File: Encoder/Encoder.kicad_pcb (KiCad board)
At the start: 2 copper layers, 158.6 x 85.2 mm, 52 parts, among them J1 Conn_01x02_Socket, J2 Conn_01x02_Socket, J3 Conn_01x04_Socket, U1 TL072, U2 TL072, U3 TL072

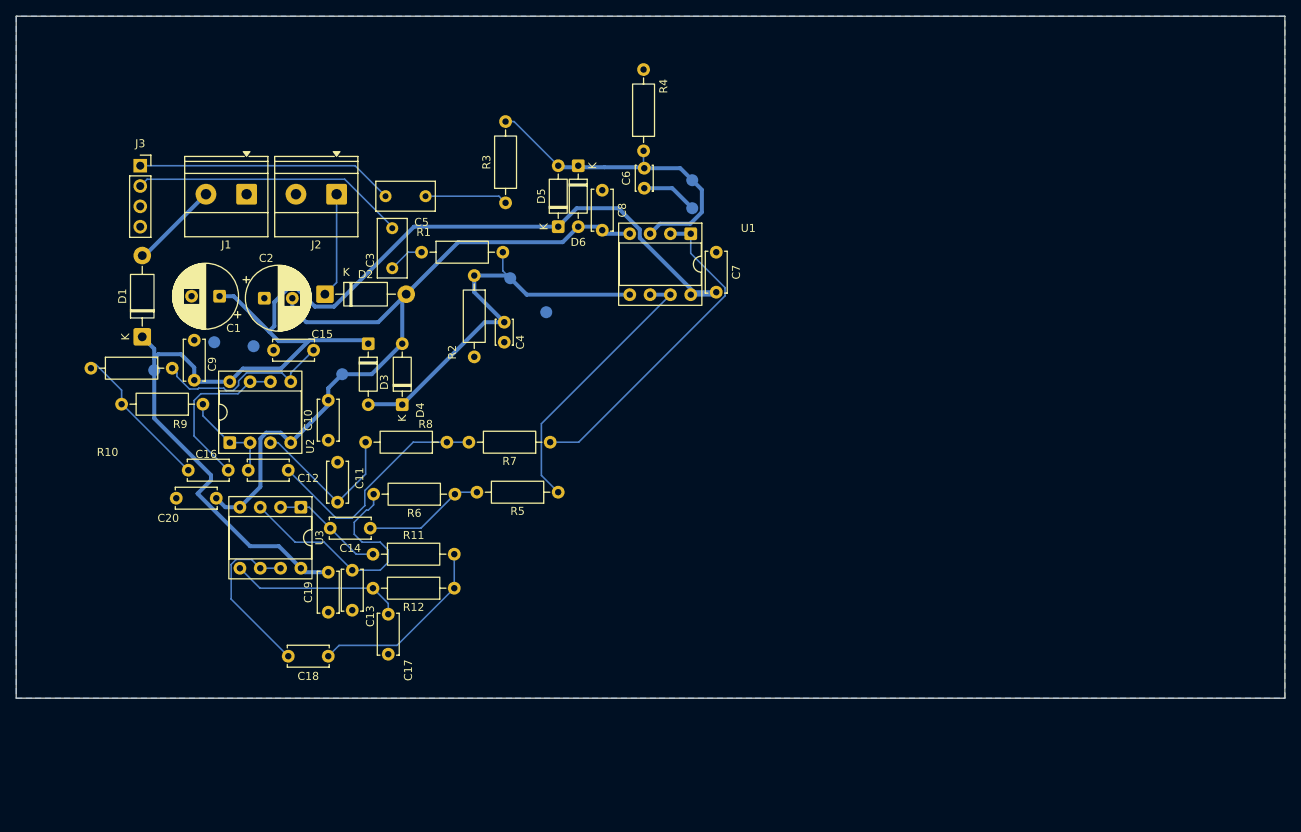
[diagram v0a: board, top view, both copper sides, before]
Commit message: new board layout
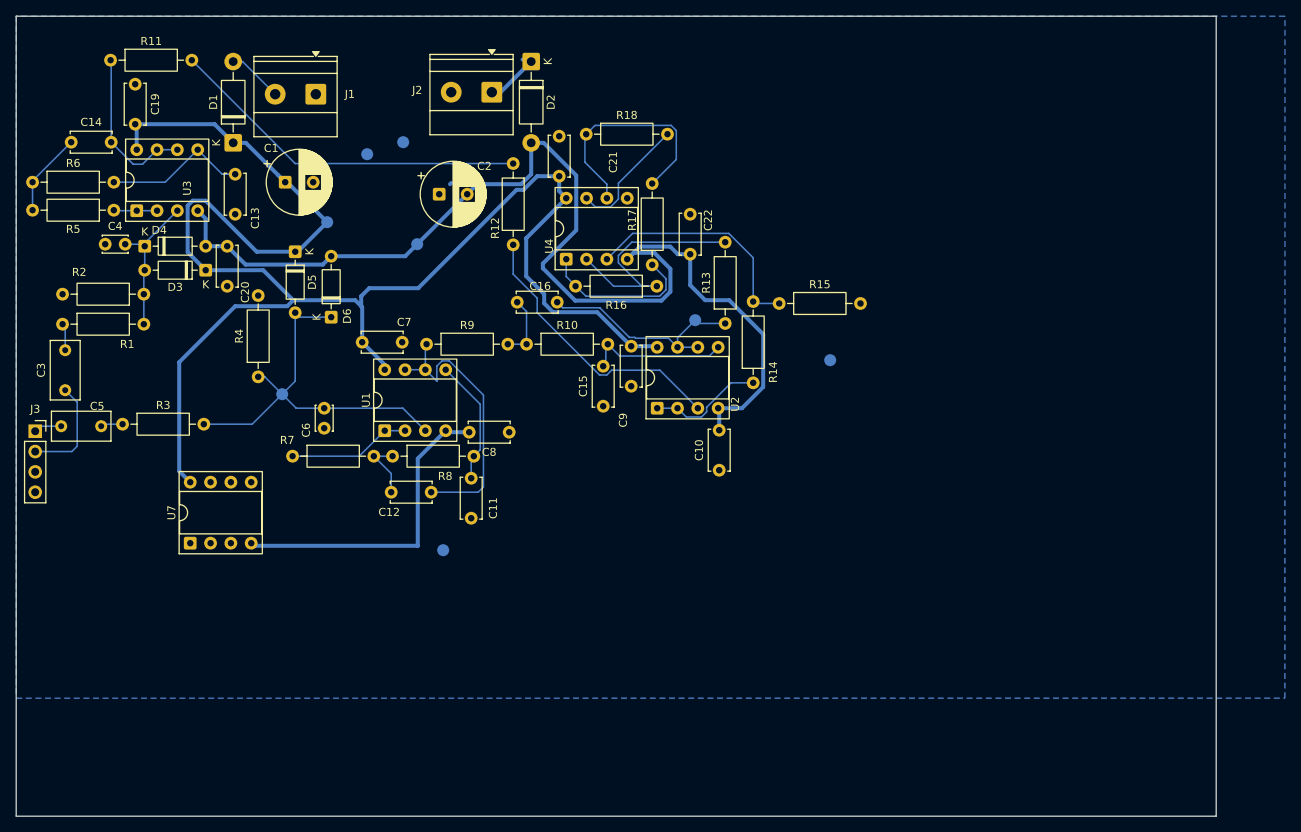
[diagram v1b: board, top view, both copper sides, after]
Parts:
- removed C17: 330 p, Capacitor_THT:C_Disc_D5.0mm_W2.5mm_P5.00mm
- removed C18: 2.2 n, Capacitor_THT:C_Disc_D5.0mm_W2.5mm_P5.00mm
- removed TP_GND2, TP_R1: TestPoint, TestPoint:TestPoint_Pad_D1.5mm
- added C21: 100n, Capacitor_THT:C_Disc_D5.0mm_W2.5mm_P5.00mm, F.Cu at (79.9, 27.0)
- added C22: 100n, Capacitor_THT:C_Disc_D5.0mm_W2.5mm_P5.00mm, F.Cu at (96.2, 36.8)
- added R13: 100k, Resistor_THT:R_Axial_DIN0207_L6.3mm_D2.5mm_P10.16mm_Horizontal, F.Cu at (100.6, 50.4)
- added R14: 100k, Resistor_THT:R_Axial_DIN0207_L6.3mm_D2.5mm_P10.16mm_Horizontal, F.Cu at (104.1, 57.8)
- added R15: 100k, Resistor_THT:R_Axial_DIN0207_L6.3mm_D2.5mm_P10.16mm_Horizontal, F.Cu at (107.4, 47.9)
- added R16: 100k, Resistor_THT:R_Axial_DIN0207_L6.3mm_D2.5mm_P10.16mm_Horizontal, F.Cu at (92.1, 45.8)
- added R17: 100k, Resistor_THT:R_Axial_DIN0207_L6.3mm_D2.5mm_P10.16mm_Horizontal, F.Cu at (91.5, 43.1)
- added R18: 100k, Resistor_THT:R_Axial_DIN0207_L6.3mm_D2.5mm_P10.16mm_Horizontal, F.Cu at (83.2, 26.8)
- added TP_GND5: TestPoint, TestPoint:TestPoint_Pad_D1.5mm, B.Cu at (113.8, 55.0)
- added TP_L2: TestPoint, TestPoint:TestPoint_Pad_D1.5mm, B.Cu at (96.9, 50.0)
- added U4: TL072, Package_DIP:DIP-8_W7.62mm_Socket, F.Cu at (80.8, 42.4)
- added U7: TL072, Package_DIP:DIP-8_W7.62mm_Socket, F.Cu at (33.8, 77.9)
- moved C19 70.3 mm to (26.9, 20.5), turned to -90 degrees
- moved R11 69.9 mm to (23.8, 17.5)
- moved R5 65.8 mm to (24.2, 36.2)
- moved R6 65.6 mm to (14.0, 32.8), turned to 0 degrees
- moved C14 61.0 mm to (18.9, 27.8), turned to 0 degrees
- moved TP_L1 57.8 mm to (45.2, 59.2), turned to 180 degrees
- moved R4 55.8 mm to (42.2, 57.1)
- moved R3 55.3 mm to (25.3, 63.0), turned to 0 degrees
- moved C9 54.9 mm to (88.9, 58.2), turned to 90 degrees
- moved R10 54.5 mm to (75.8, 53.0)
- moved U2 53.6 mm to (92.1, 61.0)
- moved R12 53.6 mm to (74.1, 30.4), turned to -90 degrees
- moved TP_GND4 52.9 mm to (65.4, 78.8), turned to 180 degrees
- moved C13 51.6 mm to (39.4, 36.8)
- moved C4 51.4 mm to (23.1, 40.5), turned to 0 degrees
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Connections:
- C11 pad 2: Net-(U2A-+) -> Net-(U1B-+)
- C12 pad 2: Net-(U2A--) -> Net-(U1B--)
- C13 pad 2: Net-(U3A-+) -> Net-(U3B-+)
- C14 pad 2: Net-(U3A--) -> Net-(U3B--)
- R11 pad 1: Net-(U3A--) -> Net-(U3B--)
- R12 pad 2: Net-(U3B-+) -> Net-(U2A-+)
- R5 pad 1: Net-(U1B--) -> Net-(U3A--)
- R6 pad 2: Net-(U3A-+) -> Net-(U3B-+)
- R8 pad 2: Net-(U2A-+) -> Net-(U1B-+)
- R9 pad 1: Net-(U2A--) -> Net-(U1B--)
- U1 pad 5: /right -> Net-(U1B-+)
- U3 pad 3: Net-(U3A-+) -> /right
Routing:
- net -9V: track 94.5 -> 183.9 mm
- net /right: track 52.8 -> 18.5 mm
- net Net-(U3A-+): track 32.4 -> 0.00 mm
- net Net-(U4A--): track 0.00 -> 31.2 mm
- net +9V: track 163.6 -> 194.7 mm
- net Net-(U4A-+): track 0.00 -> 29.7 mm
- net Net-(U4B--): track 0.00 -> 29.1 mm
- net Net-(J3-Pin_1): track 32.2 -> 3.51 mm
- net Net-(U1A--): track 41.5 -> 15.4 mm
- net Net-(C12-Pad1): track 30.1 -> 7.74 mm
- net Net-(C18-Pad1): track 23.5 -> 45.5 mm
- net Net-(J3-Pin_2): track 34.5 -> 13.1 mm
- net Net-(R16-Pad2): track 0.00 -> 19.8 mm
- net Net-(U1B-+): track 0.00 -> 15.8 mm
- net Net-(R18-Pad2): track 0.00 -> 15.5 mm
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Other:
- board size 158.6 x 85.2 mm -> 150 x 100 mm

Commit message: encoder pcb test 1 is almost done
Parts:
- removed the U2 at (92.1, 61.0)
- removed U7: TL072, Package_DIP:DIP-8_W7.62mm_Socket
- added C17: 2.2n, Capacitor_THT:C_Disc_D5.0mm_W2.5mm_P5.00mm, F.Cu at (142.2, 113.8)
- added C18: 100n, Capacitor_THT:C_Disc_D5.0mm_W2.5mm_P5.00mm, F.Cu at (134.9, 113.8)
- added C23: 1 n, Capacitor_THT:C_Disc_D5.0mm_W2.5mm_P5.00mm, F.Cu at (58.0, 57.2)
- added C24: 1 n, Capacitor_THT:C_Disc_D5.0mm_W2.5mm_P5.00mm, F.Cu at (65.8, 64.2)
- added C25: 1 n, Capacitor_THT:C_Disc_D5.0mm_W2.5mm_P5.00mm, F.Cu at (77.4, 94.7)
- added C26: 1 n, Capacitor_THT:C_Disc_D5.0mm_W2.5mm_P5.00mm, F.Cu at (67.5, 94.5)
- added C27: 100n, Capacitor_THT:C_Disc_D5.0mm_W2.5mm_P5.00mm, F.Cu at (128.0, 132.2)
- added C28: 100n, Capacitor_THT:C_Disc_D5.0mm_W2.5mm_P5.00mm, F.Cu at (112.2, 120.1)
- added C29: 100n, Capacitor_THT:C_Disc_D5.0mm_W2.5mm_P5.00mm, F.Cu at (101.6, 94.1)
- added C30: 100n, Capacitor_THT:C_Disc_D5.0mm_W2.5mm_P5.00mm, F.Cu at (116.0, 97.4)
- added C31: 330 p, Capacitor_THT:C_Disc_D5.0mm_W2.5mm_P5.00mm, F.Cu at (99.1, 53.2)
- added C32: 2.2 n, Capacitor_THT:C_Disc_D5.0mm_W2.5mm_P5.00mm, F.Cu at (74.2, 68.0)
- added C33: 330 p, Capacitor_THT:C_Disc_D5.0mm_W2.5mm_P5.00mm, F.Cu at (90.5, 80.8)
- added C34: 2.2 n, Capacitor_THT:C_Disc_D5.0mm_W2.5mm_P5.00mm, F.Cu at (78.2, 91.5)
- added C35: 3.3n, Capacitor_THT:C_Disc_D5.0mm_W2.5mm_P5.00mm, F.Cu at (146.1, 86.6)
- added C36: 220P, Capacitor_THT:C_Disc_D5.0mm_W2.5mm_P5.00mm, F.Cu at (146.2, 110.7)
- added C37: 100n, Capacitor_THT:C_Disc_D5.0mm_W2.5mm_P5.00mm, F.Cu at (128.5, 70.1)
- added C38: 100n, Capacitor_THT:C_Disc_D5.0mm_W2.5mm_P5.00mm, F.Cu at (125.8, 82.4)
- added C39: 100n, Capacitor_THT:C_Disc_D5.0mm_W2.5mm_P5.00mm, F.Cu at (129.0, 62.5)
- added C40: 100n, Capacitor_THT:C_Disc_D5.0mm_W2.5mm_P5.00mm, F.Cu at (126.3, 102.8)
- added C41: 100n, Capacitor_THT:C_Disc_D5.0mm_W2.5mm_P5.00mm, F.Cu at (132.6, 67.4)
- added R19: 100k, Resistor_THT:R_Axial_DIN0207_L6.3mm_D2.5mm_P10.16mm_Horizontal, F.Cu at (76.9, 72.8)
- added R20: 100k, Resistor_THT:R_Axial_DIN0207_L6.3mm_D2.5mm_P10.16mm_Horizontal, F.Cu at (82.9, 78.0)
- added R21: 100k, Resistor_THT:R_Axial_DIN0207_L6.3mm_D2.5mm_P10.16mm_Horizontal, F.Cu at (106.8, 78.3)
- added R22: 100k, Resistor_THT:R_Axial_DIN0207_L6.3mm_D2.5mm_P10.16mm_Horizontal, F.Cu at (94.8, 107.8)
- added R23: 100k, Resistor_THT:R_Axial_DIN0207_L6.3mm_D2.5mm_P10.16mm_Horizontal, F.Cu at (90.2, 107.7)
- added R24: 100k, Resistor_THT:R_Axial_DIN0207_L6.3mm_D2.5mm_P10.16mm_Horizontal, F.Cu at (109.4, 81.0)
- added R25: 100k, Resistor_THT:R_Axial_DIN0207_L6.3mm_D2.5mm_P10.16mm_Horizontal, F.Cu at (84.9, 106.4)
- added R26: 100k, Resistor_THT:R_Axial_DIN0207_L6.3mm_D2.5mm_P10.16mm_Horizontal, F.Cu at (111.5, 78.3)
- added R27: 100k, Resistor_THT:R_Axial_DIN0207_L6.3mm_D2.5mm_P10.16mm_Horizontal, F.Cu at (89.1, 101.4)
- added R28: 100k, Resistor_THT:R_Axial_DIN0207_L6.3mm_D2.5mm_P10.16mm_Horizontal, F.Cu at (100.8, 67.4)
- added R29: 1k, Resistor_THT:R_Axial_DIN0207_L6.3mm_D2.5mm_P10.16mm_Horizontal, F.Cu at (103.4, 61.0)
- added R30: 100k, Resistor_THT:R_Axial_DIN0207_L6.3mm_D2.5mm_P10.16mm_Horizontal, F.Cu at (85.7, 101.6)
- added R31: 51, Resistor_THT:R_Axial_DIN0207_L6.3mm_D2.5mm_P10.16mm_Horizontal, F.Cu at (113.6, 64.2)
- added R32: 51, Resistor_THT:R_Axial_DIN0207_L6.3mm_D2.5mm_P10.16mm_Horizontal, F.Cu at (103.4, 57.8)
- added R33: 6.8k, Resistor_THT:R_Axial_DIN0207_L6.3mm_D2.5mm_P10.16mm_Horizontal, F.Cu at (114.6, 68.1)
- added R34: 3.9k, Resistor_THT:R_Axial_DIN0207_L6.3mm_D2.5mm_P10.16mm_Horizontal, F.Cu at (122.7, 87.4)
- added R35: 1k, Resistor_THT:R_Axial_DIN0207_L6.3mm_D2.5mm_P10.16mm_Horizontal, F.Cu at (128.3, 73.3)
- added R36: 3.9k, Resistor_THT:R_Axial_DIN0207_L6.3mm_D2.5mm_P10.16mm_Horizontal, F.Cu at (129.0, 93.1)
- added R37: 1k, Resistor_THT:R_Axial_DIN0207_L6.3mm_D2.5mm_P10.16mm_Horizontal, F.Cu at (135.7, 78.1)
- added R38: 10k, Resistor_THT:R_Axial_DIN0207_L6.3mm_D2.5mm_P10.16mm_Horizontal, F.Cu at (136.3, 70.4)
- added R39: 15k, Resistor_THT:R_Axial_DIN0207_L6.3mm_D2.5mm_P10.16mm_Horizontal, F.Cu at (129.0, 80.7)
- added R40: 15k, Resistor_THT:R_Axial_DIN0207_L6.3mm_D2.5mm_P10.16mm_Horizontal, F.Cu at (121.8, 100.1)
- added R41: 7.5k, Resistor_THT:R_Axial_DIN0207_L6.3mm_D2.5mm_P10.16mm_Horizontal, F.Cu at (132.0, 90.9)
- added R42: 2.2k, Resistor_THT:R_Axial_DIN0207_L6.3mm_D2.5mm_P10.16mm_Horizontal, F.Cu at (135.2, 80.7)
- added R43: 15k, Resistor_THT:R_Axial_DIN0207_L6.3mm_D2.5mm_P10.16mm_Horizontal, F.Cu at (138.2, 91.1)
- added R44: 15k, Resistor_THT:R_Axial_DIN0207_L6.3mm_D2.5mm_P10.16mm_Horizontal, F.Cu at (105.0, 110.2)
- added R45: 100K, Resistor_THT:R_Axial_DIN0207_L6.3mm_D2.5mm_P10.16mm_Horizontal, F.Cu at (111.6, 110.3)
- added R46: 270K, Resistor_THT:R_Axial_DIN0207_L6.3mm_D2.5mm_P10.16mm_Horizontal, F.Cu at (108.4, 100.0)
- added R47: 360K, Resistor_THT:R_Axial_DIN0207_L6.3mm_D2.5mm_P10.16mm_Horizontal, F.Cu at (108.2, 124.4)
- added R48: 100K, Resistor_THT:R_Axial_DIN0207_L6.3mm_D2.5mm_P10.16mm_Horizontal, F.Cu at (110.9, 114.6)
- added R49: 100K, Resistor_THT:R_Axial_DIN0207_L6.3mm_D2.5mm_P10.16mm_Horizontal, F.Cu at (124.5, 109.8)
- added R50: 100K, Resistor_THT:R_Axial_DIN0207_L6.3mm_D2.5mm_P10.16mm_Horizontal, F.Cu at (127.2, 119.7)
- added TP_GND2: TestPoint, TestPoint:TestPoint_Pad_D1.5mm, F.Cu at (-69.1, 81.5)
- added TP_R1: TestPoint, TestPoint:TestPoint_Pad_D1.5mm, F.Cu at (-65.6, 85.1)
- added U10: NE5532, Package_DIP:DIP-8_W7.62mm_Socket, F.Cu at (105.0, 97.2)
- added U2: NE5532, Package_DIP:DIP-8_W7.62mm_Socket, F.Cu at (136.8, 124.6)
- added U2: TL072, Package_DIP:DIP-8_W7.62mm_Socket, F.Cu at (71.9, 83.8)
- added U5: TL072, Package_DIP:DIP-8_W7.62mm_Socket, F.Cu at (95.9, 77.8)
- added U6: TL072, Package_DIP:DIP-8_W7.62mm_Socket, F.Cu at (78.0, 117.2)
- added U8: TL072, Package_DIP:DIP-8_W7.62mm_Socket, F.Cu at (123.2, 119.4)
- added U9: MC1496, Package_DIP:DIP-14_W7.62mm_Socket, F.Cu at (118.1, 58.0)
- C1, C2: value 22u -> 1u; footprint Capacitor_THT:CP_Radial_D8.0mm_P3.50mm -> Capacitor_THT:C_Rect_L7.2mm_W3.5mm_P5.00mm
- C11, C12: value 1 n -> 100p; footprint Capacitor_THT:C_Disc_D5.0mm_W2.5mm_P5.00mm -> Capacitor_THT:C_Disc_D3.0mm_W2.0mm_P2.50mm
- C13, C14: value 1 n -> 100n
- C15: value 330 p -> 100n
- C16: value 2.2 n -> 100n
- C20: value 100n -> 1n
- C3: value 1u -> 22u; footprint Capacitor_THT:C_Rect_L7.2mm_W3.5mm_P5.00mm -> Capacitor_THT:CP_Radial_D8.0mm_P3.50mm
- C4: value 100p -> 22u; footprint Capacitor_THT:C_Disc_D3.0mm_W2.0mm_P2.50mm -> Capacitor_THT:CP_Radial_D8.0mm_P3.50mm
- C5: value 1u -> 1n; footprint Capacitor_THT:C_Rect_L7.2mm_W3.5mm_P5.00mm -> Capacitor_THT:C_Disc_D5.0mm_W2.5mm_P5.00mm
- C6: value 100p -> 1.2n; footprint Capacitor_THT:C_Disc_D3.0mm_W2.0mm_P2.50mm -> Capacitor_THT:C_Disc_D5.0mm_W2.5mm_P5.00mm
- R1, R5: value 10k -> 2.4k
- R10, R11, R12, R9: value 12k -> 10k
- R13, R14, R15, R17: value 100k -> 12k
- R16, R18: value 100k -> 3.3k
- R2: value 100k -> 10k
- R6: value 10k -> 100k
- R7, R8: value 10k -> 1.8k
- TP_+9V1, TP_-9V1, TP_GND1, TP_GND3, TP_GND4, TP_GND5, TP_L1, TP_L2: moved to F.Cu
- moved TP_GND5 180.4 mm to (-65.6, 74.4), turned to 0 degrees
- moved TP_L2 165.5 mm to (-65.6, 81.5), turned to 0 degrees
- moved C19 158.9 mm to (144.6, 127.2)
- moved TP_GND1 138.9 mm to (-69.1, 78.0), turned to 0 degrees
- moved TP_GND3 136.9 mm to (-69.1, 85.1), turned to 0 degrees
- moved TP_-9V1 135.6 mm to (-69.1, 74.4), turned to 0 degrees
- moved R5 131.3 mm to (136.6, 104.1), turned to 90 degrees
- moved TP_GND4 131.2 mm to (-65.6, 70.9), turned to 0 degrees
- moved C5 126.1 mm to (139.8, 94.4)
- moved TP_+9V1 124.5 mm to (-69.1, 70.9), turned to 0 degrees
- moved R1 122.7 mm to (126.8, 106.8)
- moved TP_L1 112.4 mm to (-65.6, 78.0), turned to 0 degrees
- moved J1 110.3 mm to (79.2, 127.9), turned to 0 degrees
- moved D1 109.3 mm to (74.0, 131.4)
- moved C20 107.7 mm to (141.4, 77.0), turned to -90 degrees
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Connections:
- C1 pad 1: +9V -> Net-(J3-Pin_1)
- C1 pad 2: GND -> Net-(C1-Pad2)
- C11 pad 2: Net-(U1B-+) -> /left
- C12 pad 1: Net-(C12-Pad1) -> GND
- C12 pad 2: Net-(U1B--) -> /right
- C13 pad 2: Net-(U3B-+) -> +9V
- C14 pad 1: Net-(C14-Pad1) -> GND
- C14 pad 2: Net-(U3B--) -> -9V
- C15 pad 2: Net-(U2B-+) -> +9V
- C16 pad 1: Net-(C16-Pad1) -> GND
- C16 pad 2: Net-(U2B--) -> -9V
- C19 pad 1: GND -> -9V
- C19 pad 2: +9V -> GND
- C2 pad 1: GND -> Net-(J3-Pin_2)
- C2 pad 2: -9V -> Net-(C2-Pad2)
- C20 pad 2: -9V -> Net-(U2A--)
- C22 pad 1: GND -> -9V
- C22 pad 2: -9V -> GND
- C3 pad 1: Net-(J3-Pin_2) -> GND
- C3 pad 2: Net-(C3-Pad2) -> -9V
- C4 pad 1: GND -> +9V
- C4 pad 2: /right -> GND
- C5 pad 1: Net-(J3-Pin_1) -> Net-(U10B-+)
- C5 pad 2: Net-(C5-Pad2) -> GND
- C6 pad 1: GND -> Net-(C6-Pad1)
- C6 pad 2: /left -> Net-(U10B--)
- D1 pad 1: +9V -> Net-(D1-K)
- D1 pad 2: Net-(D1-A) -> -9V
- D2 pad 1: Net-(D2-K) -> +9V
- D2 pad 2: -9V -> Net-(D2-A)
- D3 pad 2: /right -> /left
- D4 pad 1: /right -> /left
- D5 pad 2: /left -> /right
- D6 pad 1: /left -> /right
- J1 pad 1: GND -> Net-(D1-K)
- J1 pad 2: Net-(D1-A) -> GND
- J2 pad 1: Net-(D2-K) -> GND
- J2 pad 2: GND -> Net-(D2-A)
- R1 pad 1: Net-(C3-Pad2) -> Net-(R1-Pad1)
- R1 pad 2: /right -> Net-(C6-Pad1)
- R10 pad 1: Net-(C16-Pad1) -> Net-(U3A--)
- R10 pad 2: Net-(U2B-+) -> Net-(C26-Pad1)
- R11 pad 1: Net-(U3B--) -> Net-(C24-Pad1)
- R11 pad 2: Net-(C18-Pad1) -> Net-(U1B-+)
- R12 pad 1: Net-(C18-Pad1) -> Net-(C26-Pad1)
- R12 pad 2: Net-(U2A-+) -> Net-(U3B-+)
- R13 pad 1: Net-(U2B--) -> Net-(U1B--)
- R13 pad 2: Net-(U4A--) -> Net-(C32-Pad1)
- R14 pad 1: Net-(U2A--) -> Net-(C32-Pad1)
- R14 pad 2: Net-(U4A-+) -> Net-(U4B-+)
- R15 pad 1: Net-(U4A-+) -> Net-(U3B--)
- R15 pad 2: GND -> Net-(C34-Pad1)
- R16 pad 1: Net-(U4A--) -> Net-(U2A-+)
- R16 pad 2: Net-(R16-Pad2) -> Net-(C35-Pad1)
- R17 pad 1: Net-(R16-Pad2) -> Net-(C34-Pad1)
- R17 pad 2: Net-(U4B--) -> Net-(U4A-+)
- R18 pad 1: Net-(U4B--) -> Net-(C35-Pad1)
- R18 pad 2: Net-(R18-Pad2) -> Net-(U2B--)
- R2 pad 1: /right -> Net-(C1-Pad2)
- R2 pad 2: GND -> /left
- R3 pad 1: Net-(C5-Pad2) -> Net-(C2-Pad2)
- R3 pad 2: /left -> /right
- R5 pad 1: Net-(U3A--) -> Net-(C6-Pad1)
- R5 pad 2: Net-(C14-Pad1) -> Net-(U10B-+)
- R6 pad 1: Net-(C14-Pad1) -> /right
- R6 pad 2: Net-(U3B-+) -> GND
- R7 pad 1: Net-(U1A--) -> Net-(U10B--)
- R7 pad 2: Net-(C12-Pad1) -> Net-(C17-Pad1)
- R8 pad 1: Net-(C12-Pad1) -> Net-(C17-Pad1)
- R8 pad 2: Net-(U1B-+) -> Net-(U2A--)
- R9 pad 1: Net-(U1B--) -> Net-(U1A--)
- R9 pad 2: Net-(C16-Pad1) -> Net-(C24-Pad1)
- TP_L2 pad 1: Net-(U2B--) -> Net-(U4B--)
- U4 pad 1: Net-(R16-Pad2) -> Net-(U4A--)
- U4 pad 5: GND -> Net-(U4B-+)
- U4 pad 7: Net-(R18-Pad2) -> Net-(U4B--)
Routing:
- net -9V: track 183.9 -> 330.0 mm
- net Net-(U2A--): track 14.6 -> 139.0 mm, vias 0 -> 1
- net +9V: track 194.7 -> 306.4 mm, vias 0 -> 1
- net Net-(U2B-+): track 18.0 -> 115.4 mm, vias 0 -> 1
- net Net-(U2A-+): track 35.2 -> 124.3 mm, vias 0 -> 1
- net Net-(U2B--): track 28.1 -> 95.4 mm, vias 0 -> 2
- net Net-(C18-Pad1): track 45.5 -> 0.00 mm
- net Net-(U9-VO-): track 0.00 -> 45.5 mm
- net Net-(U4B--): track 29.1 -> 71.7 mm, vias 0 -> 1
- net Net-(U10A--): track 0.00 -> 42.4 mm
- net Net-(R30-Pad2): track 0.00 -> 42.3 mm
- net Net-(R48-Pad2): track 0.00 -> 39.1 mm
- net Net-(U10B--): track 0.00 -> 37.9 mm, vias 0 -> 1
- net Net-(U8B--): track 0.00 -> 37.2 mm
- net /right: track 18.5 -> 55.2 mm
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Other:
- board size 150 x 100 mm -> 120 x 100 mm
